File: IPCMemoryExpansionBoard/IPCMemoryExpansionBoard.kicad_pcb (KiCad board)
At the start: 2 copper layers, 185 x 116 mm, 112 parts, among them J1 C64AC, J10 TESTPOINTS, J11 TESTPOINTS, J12 TESTPOINTS, J13 TESTPOINT, J14 TESTPOINT, J15 TESTPOINT, J16 TESTPOINT, J17 TESTPOINT, J18 TESTPOINT, J19 TESTPOINT, J2 TESTPOINTS, J20 TESTPOINT, J21 TESTPOINT, J22 TESTPOINT, J23 TESTPOINT, J24 TESTPOINT, J25 TESTPOINT, J26 TESTPOINT, J27 TESTPOINT, J28 TESTPOINT, J29 TESTPOINT, J3 USB_B_Micro, J4 JTAG, J5 JTAG-STM32, J6 SERIAL, J7 TESTPOINTS, J8 TESTPOINTS, J9 TESTPOINTS, SW1 CONFIG SWITCH, U1 74LVC245, U10 74LVC245, U11 74LS38, U13 AMS1117-3.3, U2 74LVC245, U3 74LVC245, U4 74LVC245, U5 74LVC245, U6 XC2C32A, U7 SST38VF6401, U8 AS6C6416, U9 STM32F407ZETx, Y1 8MHz

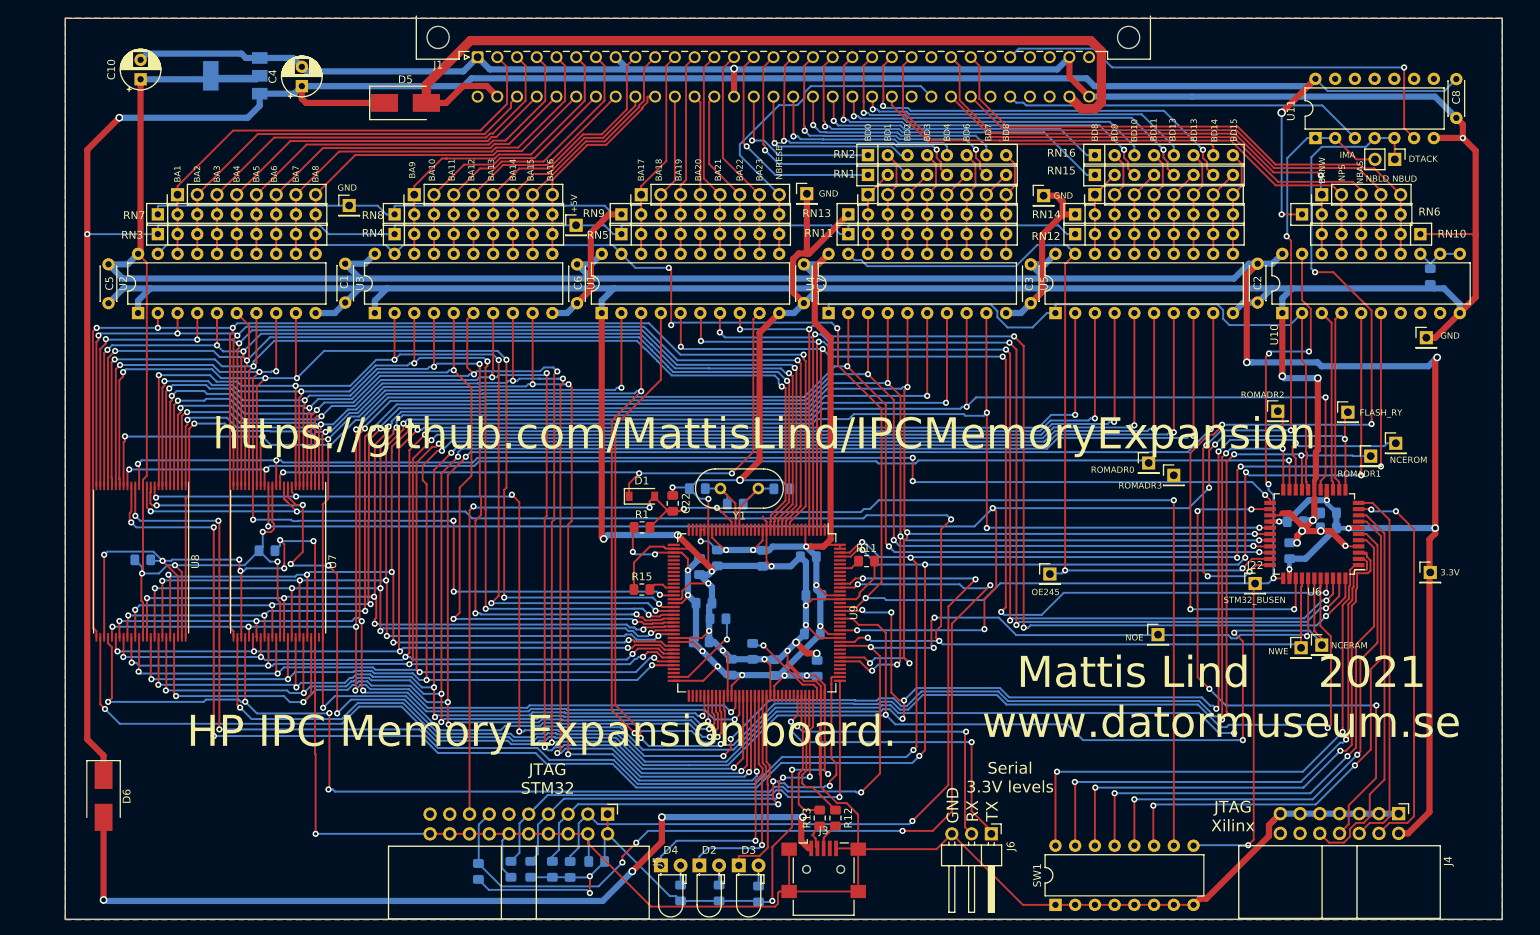
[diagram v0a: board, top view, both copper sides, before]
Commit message: Layout ready.
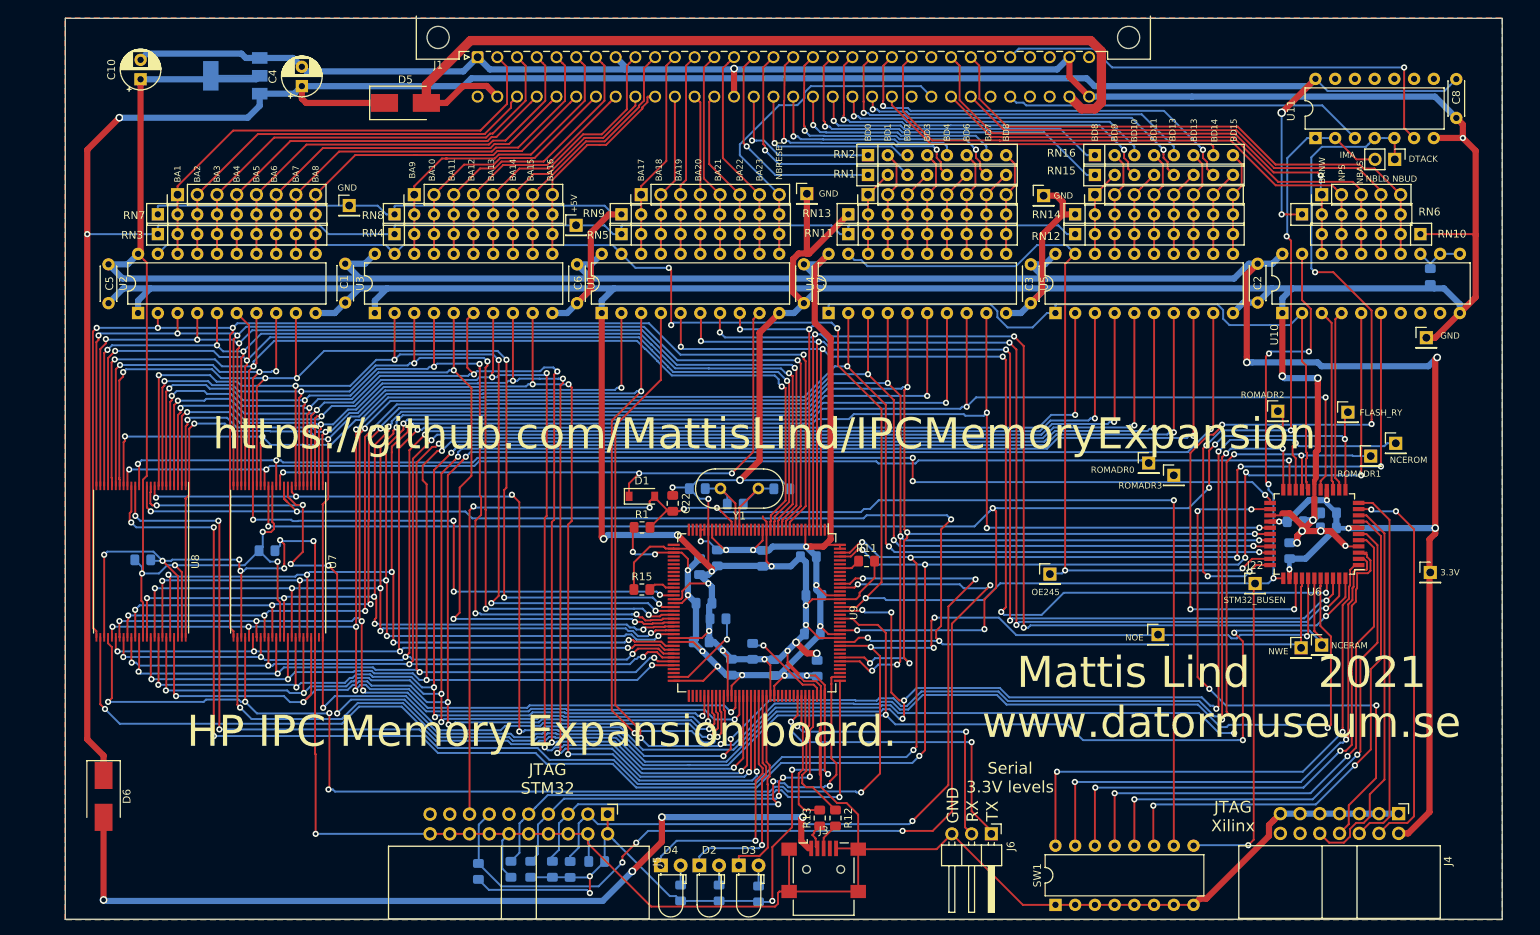
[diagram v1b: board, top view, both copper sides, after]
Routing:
- added copper zone on B.Cu, net +3V3
- removed copper zone on B.Cu, net GND
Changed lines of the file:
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@@
     (polygon
       (pts
-        (xy 215.011 29.972) (xy 29.972 29.972) (xy 29.972 146.05) (xy 215.011 146.05)
+        (xy 29.972 29.972) (xy 215.011 29.972) (xy 215.011 146.05) (xy 29.972 146.05)
       )
     )
   )
-  (zone (net 2) (net_name GND) (layer B.Cu) (hatch edge 0.508)
+  (zone (net 1) (net_name +3V3) (layer B.Cu) (hatch edge 0.508)
     (connect_pads (clearance 0.508))
     (min_thickness 0.254)
